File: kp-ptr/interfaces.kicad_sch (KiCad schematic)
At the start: 10 parts

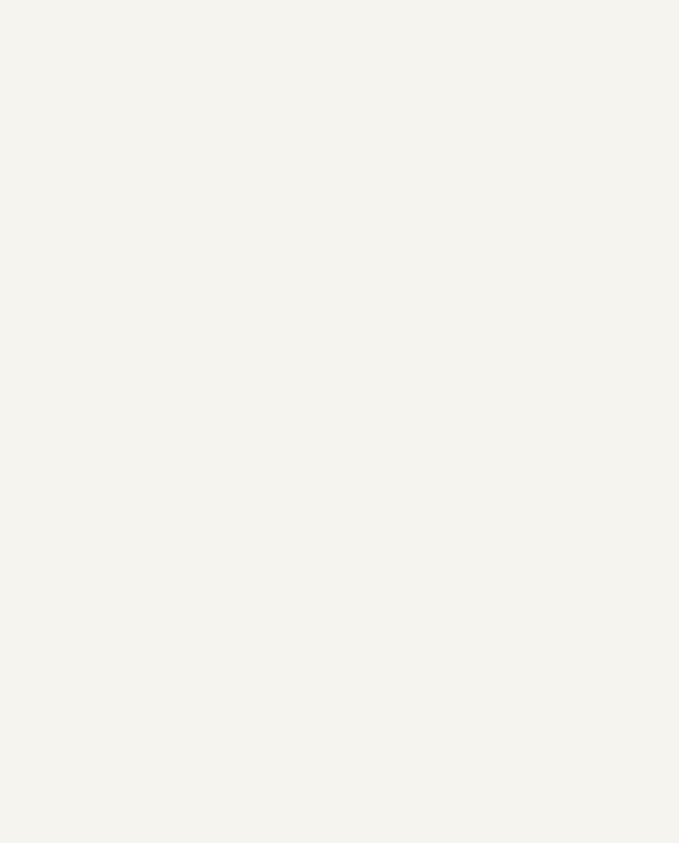
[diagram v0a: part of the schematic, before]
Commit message: GPS lora wrzucone symbole Signed-off-by: kretu <krecik@gmail.com>
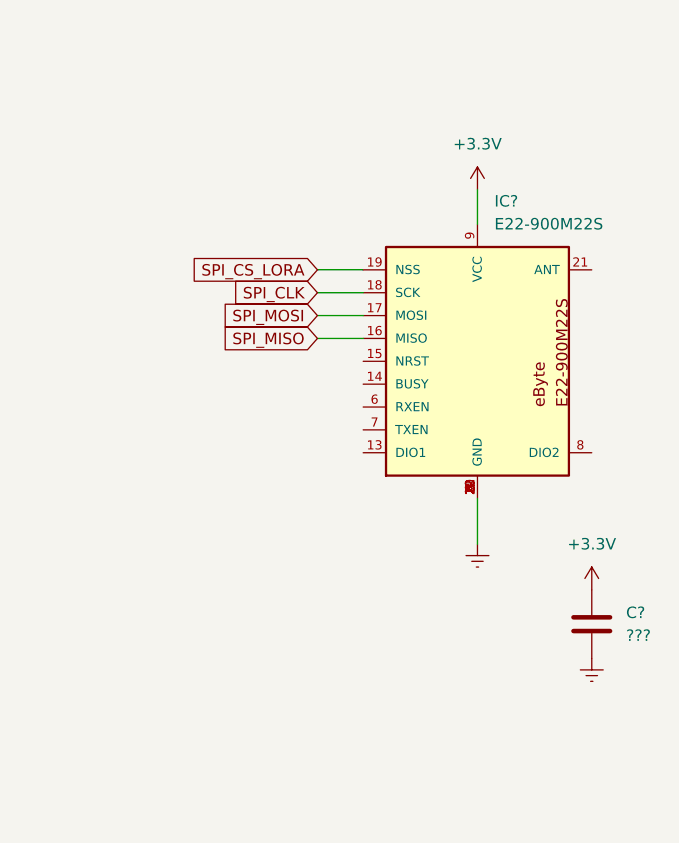
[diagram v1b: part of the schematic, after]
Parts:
- added C?: ???, symbol Device:C
- added IC?: E22-900M22S, E22-900M22S, symbol KP-PTR_lib:E22-900M22S
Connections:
- net +3V3: now also C?.1, IC?.9 (VCC)
- net Earth: now also C?.2, IC?.1 (GND), IC?.10 (GND), IC?.11 (GND), IC?.12 (GND), IC?.2 (GND), IC?.20 (GND), IC?.22 (GND), IC?.3 (GND), IC?.4 (GND), IC?.5 (GND)
- net SPI_CLK: now also IC?.18 (SCK)
- net SPI_MISO: now also IC?.16 (MISO)
- net SPI_MOSI: now also IC?.17 (MOSI)
- new net SPI_CS_LORA: IC?.19 (NSS)
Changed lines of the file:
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@@
   (junction (at 57.15 110.49) (diameter 0) (color 0 0 0 0)
   )
+  (wire (pts (xy 222.25 33.02) (xy 222.25 36.83))
+    (stroke (width 0) (type default) (color 0 0 0 0))
+  )
   (wire (pts (xy 57.15 97.79) (xy 66.04 97.79))
     (stroke (width 0) (type default) (color 0 0 0 0))
@@
     (stroke (width 0) (type default) (color 0 0 0 0))
   )
+  (wire (pts (xy 204.47 46.99) (xy 209.55 46.99))
+    (stroke (width 0) (type default) (color 0 0 0 0))
+  )
   (wire (pts (xy 68.58 38.1) (xy 63.5 38.1))
     (stroke (width 0) (type default) (color 0 0 0 0))
@@
     (stroke (width 0) (type default) (color 0 0 0 0))
   )
+  (wire (pts (xy 222.25 72.39) (xy 222.25 67.31))
+    (stroke (width 0) (type default) (color 0 0 0 0))
+  )
   (wire (pts (xy 57.15 102.87) (xy 57.15 100.33))
     (stroke (width 0) (type default) (color 0 0 0 0))
@@
     (stroke (width 0) (type default) (color 0 0 0 0))
   )
+  (wire (pts (xy 204.47 41.91) (xy 209.55 41.91))
+    (stroke (width 0) (type default) (color 0 0 0 0))
+  )
   (wire (pts (xy 105.41 107.95) (xy 114.3 107.95))
     (stroke (width 0) (type default) (color 0 0 0 0))
@@
     (stroke (width 0) (type default) (color 0 0 0 0))
   )
+  (wire (pts (xy 204.47 49.53) (xy 209.55 49.53))
+    (stroke (width 0) (type default) (color 0 0 0 0))
+  )
   (wire (pts (xy 109.22 46.99) (xy 109.22 38.1))
     (stroke (width 0) (type default) (color 0 0 0 0))
@@
   )
   (wire (pts (xy 83.82 46.99) (xy 68.58 46.99))
+    (stroke (width 0) (type default) (color 0 0 0 0))
+  )
+  (wire (pts (xy 204.47 44.45) (xy 209.55 44.45))
     (stroke (width 0) (type default) (color 0 0 0 0))
   )
@@
     )
   )
+  (global_label "SPI_CLK" (shape input) (at 204.47 44.45 180) (fields_autoplaced)
+    (effects (font (size 1.27 1.27)) (justify right))
+    (property "Intersheet References" "${INTERSHEET_REFS}" (id 0) (at 194.4369 44.3706 0)
+      (effects (font (size 1.27 1.27)) (justify right) hide)
+    )
+  )
   (global_label "SPI_MOSI" (shape input) (at 87.63 85.09 90) (fields_autoplaced)
     (effects (font (size 1.27 1.27)) (justify left))
@@
     )
   )
+  (global_label "SPI_CS_LORA" (shape input) (at 204.47 41.91 180) (fields_autoplaced)
+    (effects (font (size 1.27 1.27)) (justify right))
+    (property "Intersheet References" "${INTERSHEET_REFS}" (id 0) (at 189.8407 41.8306 0)
+      (effects (font (size 1.27 1.27)) (justify right) hide)
+    )
+  )
   (global_label "SPI_CS_SDCARD" (shape input) (at 90.17 85.09 90) (fields_autoplaced)
     (effects (font (size 1.27 1.27)) (justify left))
     (property "Intersheet References" "${INTERSHEET_REFS}" (id 0) (at 90.2494 67.7998 90)
       (effects (font (size 1.27 1.27)) (justify left) hide)
+    )
+  )
+  (global_label "SPI_MOSI" (shape input) (at 204.47 46.99 180) (fields_autoplaced)
+    (effects (font (size 1.27 1.27)) (justify right))
+    (property "Intersheet References" "${INTERSHEET_REFS}" (id 0) (at 193.4088 46.9106 0)
+      (effects (font (size 1.27 1.27)) (justify right) hide)
+    )
+  )
+  (global_label "SPI_MISO" (shape input) (at 204.47 49.53 180) (fields_autoplaced)
+    (effects (font (size 1.27 1.27)) (justify right))
+    (property "Intersheet References" "${INTERSHEET_REFS}" (id 0) (at 193.4088 49.4506 0)
+      (effects (font (size 1.27 1.27)) (justify right) hide)
     )
   )
@@
     (pin "1")
   )
+  (symbol (lib_id "power:Earth") (at 234.95 85.09 0) (unit 1)
+    (in_bom yes) (on_board yes) (fields_autoplaced)
+    (property "Reference" "#PWR?" (id 0) (at 234.95 91.44 0)
+      (effects (font (size 1.27 1.27)) hide)
+    )
+    (property "Value" "Earth" (id 1) (at 234.95 88.9 0)
+      (effects (font (size 1.27 1.27)) hide)
+    )
+    (property "Footprint" "" (id 2) (at 234.95 85.09 0)
+      (effects (font (size 1.27 1.27)) hide)
+    )
+    (property "Datasheet" "~" (id 3) (at 234.95 85.09 0)
+      (effects (font (size 1.27 1.27)) hide)
+    )
+    (pin "1")
+  )
   (symbol (lib_id "power:Earth") (at 138.43 58.42 0) (unit 1)
     (in_bom yes) (on_board yes) (fields_autoplaced)
@@
     )
     (property "Datasheet" "~" (id 3) (at 138.43 58.42 0)
+      (effects (font (size 1.27 1.27)) hide)
+    )
+    (pin "1")
+  )
+  (symbol (lib_id "power:Earth") (at 222.25 72.39 0) (unit 1)
+    (in_bom yes) (on_board yes) (fields_autoplaced)
+    (property "Reference" "#PWR?" (id 0) (at 222.25 78.74 0)
+      (effects (font (size 1.27 1.27)) hide)
+    )
+    (property "Value" "Earth" (id 1) (at 222.25 76.2 0)
+      (effects (font (size 1.27 1.27)) hide)
+    )
+    (property "Footprint" "" (id 2) (at 222.25 72.39 0)
+      (effects (font (size 1.27 1.27)) hide)
+    )
+    (property "Datasheet" "~" (id 3) (at 222.25 72.39 0)
       (effects (font (size 1.27 1.27)) hide)
     )
@@
     (pin "2")
   )
+  (symbol (lib_id "power:+3.3V") (at 234.95 77.47 0) (unit 1)
+    (in_bom yes) (on_board yes) (fields_autoplaced)
+    (property "Reference" "#PWR?" (id 0) (at 234.95 81.28 0)
+      (effects (font (size 1.27 1.27)) hide)
+    )
+    (property "Value" "+3.3V" (id 1) (at 234.95 72.39 0))
+    (property "Footprint" "" (id 2) (at 234.95 77.47 0)
+      (effects (font (size 1.27 1.27)) hide)
+    )
+    (property "Datasheet" "" (id 3) (at 234.95 77.47 0)
+      (effects (font (size 1.27 1.27)) hide)
+    )
+    (pin "1")
+  )
   (symbol (lib_id "power:Earth") (at 130.81 58.42 0) (unit 1)
     (in_bom yes) (on_board yes) (fields_autoplaced)
@@
     )
     (pin "1")
+  )
+  (symbol (lib_id "Device:C") (at 234.95 81.28 0) (unit 1)
+    (in_bom yes) (on_board yes) (fields_autoplaced)
+    (property "Reference" "C?" (id 0) (at 238.76 80.0099 0)
+      (effects (font (size 1.27 1.27)) (justify left))
+    )
+    (property "Value" "???" (id 1) (at 238.76 82.5499 0)
+      (effects (font (size 1.27 1.27)) (justify left))
+    )
+    (property "Footprint" "" (id 2) (at 235.9152 85.09 0)
+      (effects (font (size 1.27 1.27)) hide)
+    )
+    (property "Datasheet" "~" (id 3) (at 234.95 81.28 0)
+      (effects (font (size 1.27 1.27)) hide)
+    )
+    (pin "1")
+    (pin "2")
+  )
+  (symbol (lib_id "KP-PTR_lib:E22-900M22S") (at 222.25 52.07 0) (unit 1)
+    (in_bom yes) (on_board yes) (fields_autoplaced)
+    (property "Reference" "IC?" (id 0) (at 224.1297 34.29 0)
+      (effects (font (size 1.27 1.27)) (justify left))
+    )
+    (property "Value" "E22-900M22S" (id 1) (at 224.1297 36.83 0)
+      (effects (font (size 1.27 1.27)) (justify left))
+    )
+    (property "Footprint" "E22-900M22S" (id 2) (at 222.25 52.07 0)
+      (effects (font (size 1.27 1.27)) (justify left bottom) hide)
+    )
+    (property "Datasheet" "" (id 3) (at 222.25 52.07 0)
+      (effects (font (size 1.27 1.27)) (justify left bottom) hide)
+    )
+    (pin "1")
+    (pin "10")
+    (pin "11")
+    (pin "12")
+    (pin "13")
+    (pin "14")
+    (pin "15")
+    (pin "16")
+    (pin "17")
+    (pin "18")
+    (pin "19")
+    (pin "2")
+    (pin "20")
+    (pin "21")
+    (pin "22")
+    (pin "3")
+    (pin "4")
+    (pin "5")
+    (pin "6")
+    (pin "7")
+    (pin "8")
+    (pin "9")
   )
   (symbol (lib_id "power:VBUS") (at 73.66 36.83 0) (unit 1)
@@
     (pin "2")
   )
+  (symbol (lib_id "power:+3.3V") (at 222.25 33.02 0) (unit 1)
+    (in_bom yes) (on_board yes) (fields_autoplaced)
+    (property "Reference" "#PWR?" (id 0) (at 222.25 36.83 0)
+      (effects (font (size 1.27 1.27)) hide)
+    )
+    (property "Value" "+3.3V" (id 1) (at 222.25 27.94 0))
+    (property "Footprint" "" (id 2) (at 222.25 33.02 0)
+      (effects (font (size 1.27 1.27)) hide)
+    )
+    (property "Datasheet" "" (id 3) (at 222.25 33.02 0)
+      (effects (font (size 1.27 1.27)) hide)
+    )
+    (pin "1")
+  )
   (symbol (lib_id "power:+3.3V") (at 57.15 91.44 0) (unit 1)
